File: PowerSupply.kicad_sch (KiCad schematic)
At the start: 32 parts, among them J1 Screw_Terminal_01x02, U3 LT3045xDD, U4 TLV75533PDRV, U5 LM7815, U6 LM7805_TO220

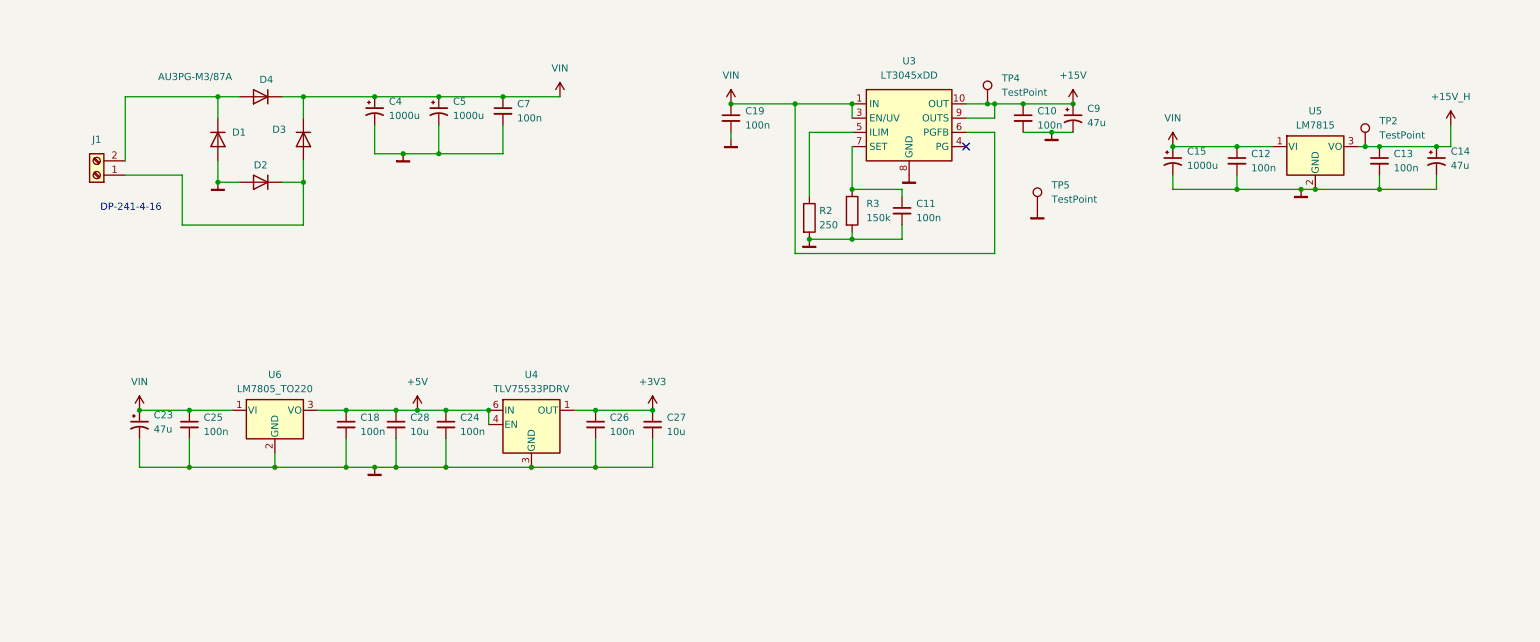
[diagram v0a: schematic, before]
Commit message: Final Version
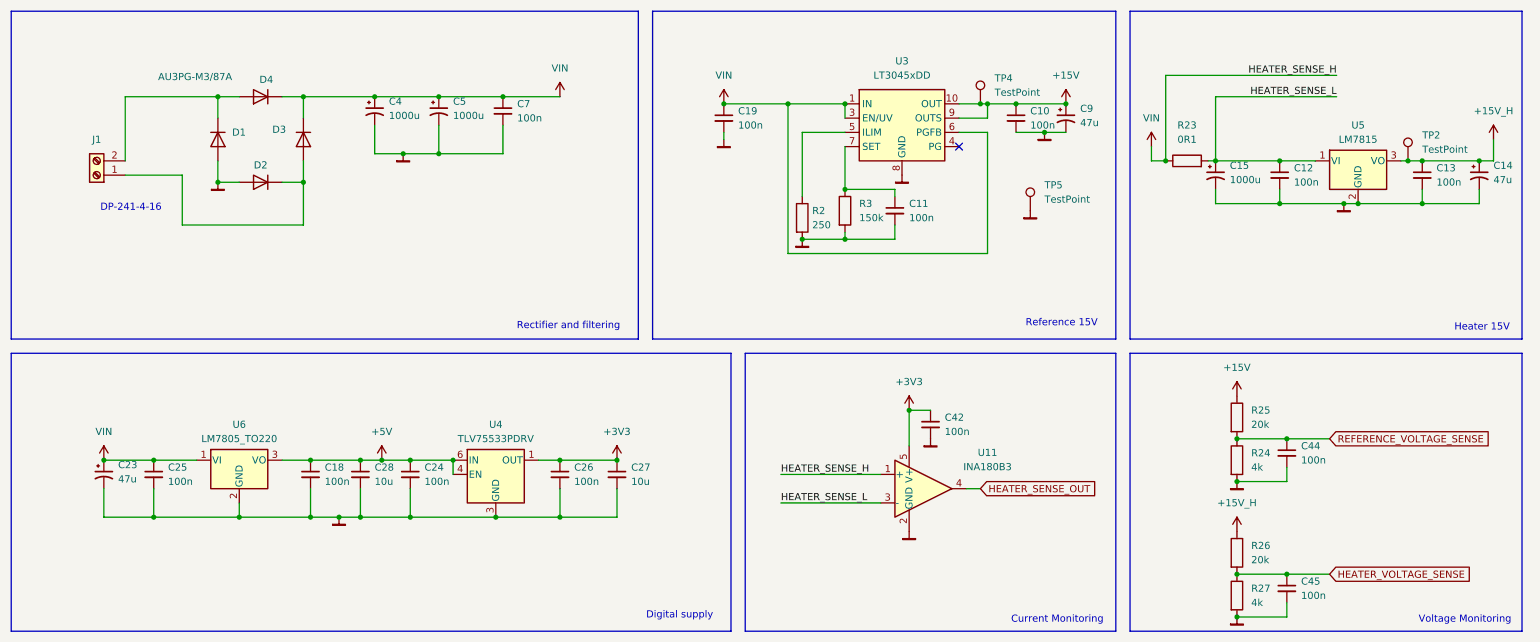
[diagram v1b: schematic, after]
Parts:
- added C42, C44, C45: 100n, Capacitor_SMD:C_0603_1608Metric, symbol Device:C_Small
- added R23: 0R1, Resistor_SMD:R_0805_2012Metric, symbol Device:R
- added R24, R27: 4k, Resistor_SMD:R_0603_1608Metric, symbol Device:R
- added R25, R26: 20k, Resistor_SMD:R_0603_1608Metric, symbol Device:R
- added U11: INA180B3, Package_TO_SOT_SMD:SOT-23-5, symbol Amplifier_Current:INA180B3
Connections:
- net +15V: now also R25.1
- net +15V_H: now also R26.1
- net +3V3: now also C42.1, U11.5 (V+)
- net Masa: now also C42.2, C44.2, C45.2, R24.2, R27.2, U11.2 (GND)
- net VIN: now also R23.1, U11.1 (+); no longer C12.1, C15.1, U5.1 (VI)
- new net HEATER_SENSE_L: C12.1, C15.1, R23.2, U11.3 (-), U5.1 (VI)
- new net HEATER_SENSE_OUT: U11.4
- new net HEATER_VOLTAGE_SENSE: C45.1, R26.2, R27.1
- new net REFERENCE_VOLTAGE_SENSE: C44.1, R24.1, R25.2
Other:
- note added: "Current Monitoring"
- note added: "Digital supply"
- note added: "Heater 15V"
- note added: "Rectifier and filtering"
- note added: "Reference 15V"
- note added: "Voltage Monitoring"
- moved on the sheet: C10, C11, C12, C13, C14, C15, C18, C19, C23, C24, C25, C26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

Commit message: Added BOM
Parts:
- C27, C28: Price (none) -> 1,51zł
- D1, D2, D3, D4: Price (none) -> 29.4zł
- R23: Price (none) -> 0,76zł
- U11: Price (none) -> 2,28zł
- U3: Price (none) -> 33,14zł
- U4: Price (none) -> 1,63zł

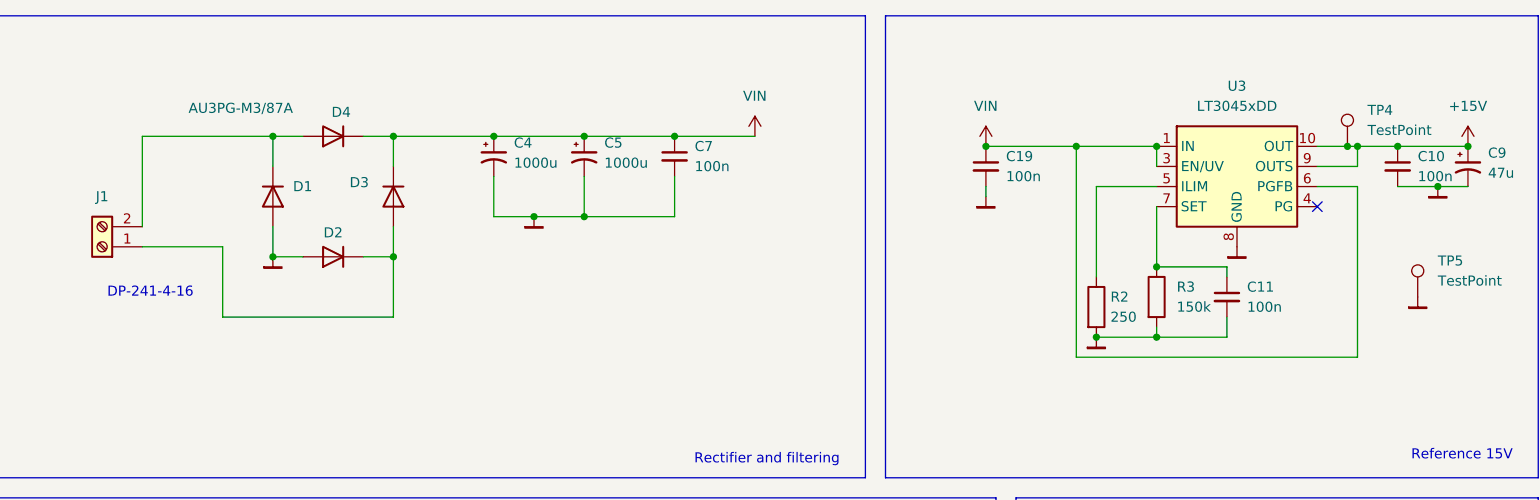
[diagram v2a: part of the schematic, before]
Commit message: Commit
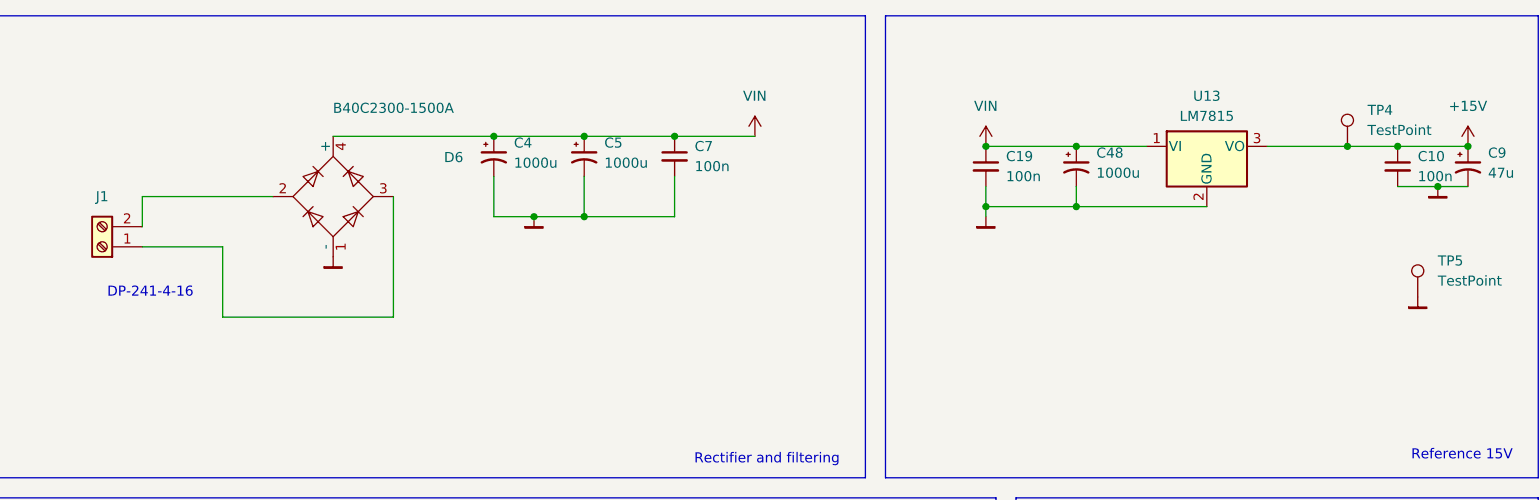
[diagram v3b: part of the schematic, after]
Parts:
- removed C11: 100n, Capacitor_SMD:C_0603_1608Metric, symbol Device:C_Small
- removed D1, D2, D3, D4: AU3PG-M3/87A, Package_TO_SOT_SMD:TO-277A, symbol Device:D
- removed R2: 250, Resistor_SMD:R_0603_1608Metric, symbol Device:R
- removed R3: 150k, Resistor_SMD:R_0603_1608Metric, symbol Device:R
- removed U3: LT3045xDD, Package_DFN_QFN:DFN-10-1EP_3x3mm_P0.5mm_EP1.65x2.38mm, symbol Regulator_Linear:LT3045xDD
- added C48: 1000u, Capacitor_THT:CP_Radial_D10.0mm_P3.80mm, symbol Device:C_Polarized_Small_US
- added D6: B40C2300-1500A, Diode_THT:Diode_Bridge_19.0x3.5x10.0mm_P5.0mm, symbol Diode_Bridge:B40C2300-1500A
- added U13: LM7815, Package_TO_SOT_THT:TO-220-3_Vertical, symbol Regulator_Linear:LM7815_TO220
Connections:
- net +15V: now also U13.3 (VO)
- net Masa: now also C48.2, D6.1 (-), U13.2 (GND)
- net VIN: now also C48.1, D6.4 (+), U13.1 (VI)
- net at J1.2 (Pin_2): now also D6.2
- net at J1.1 (Pin_1): now also D6.3
- no-connect marks 1 -> 0
